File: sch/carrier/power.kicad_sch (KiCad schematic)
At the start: 0 parts

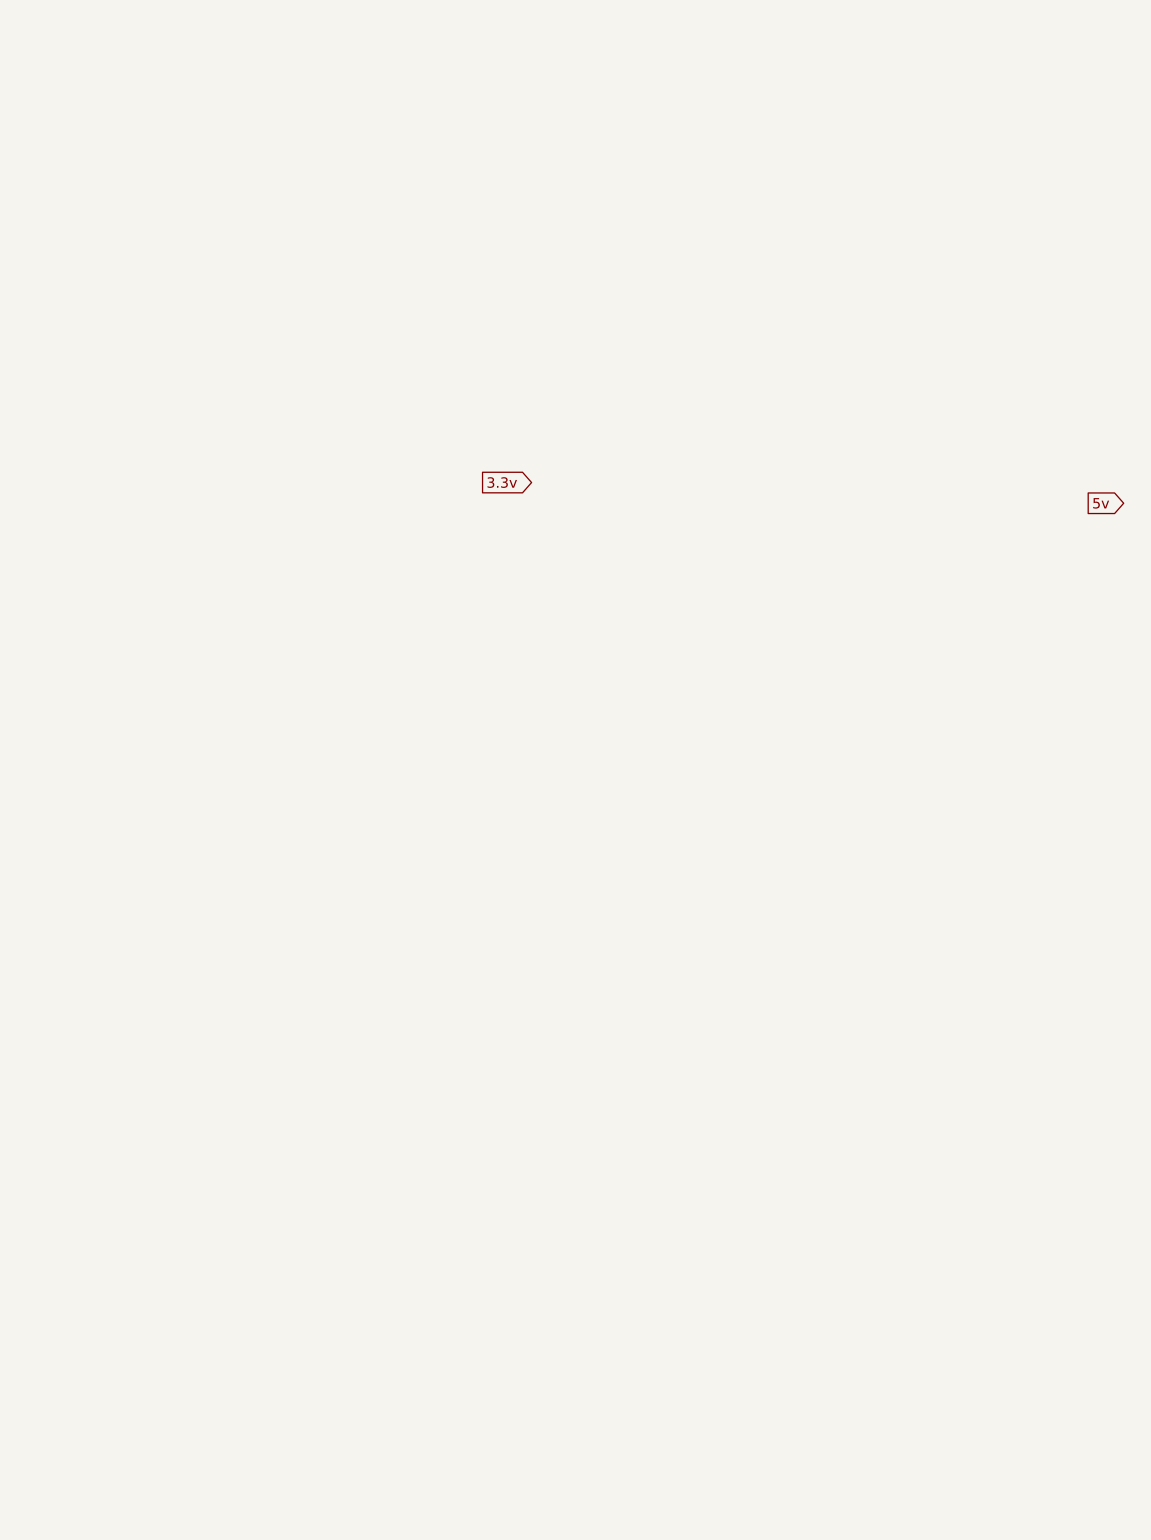
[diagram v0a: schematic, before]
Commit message: noice.
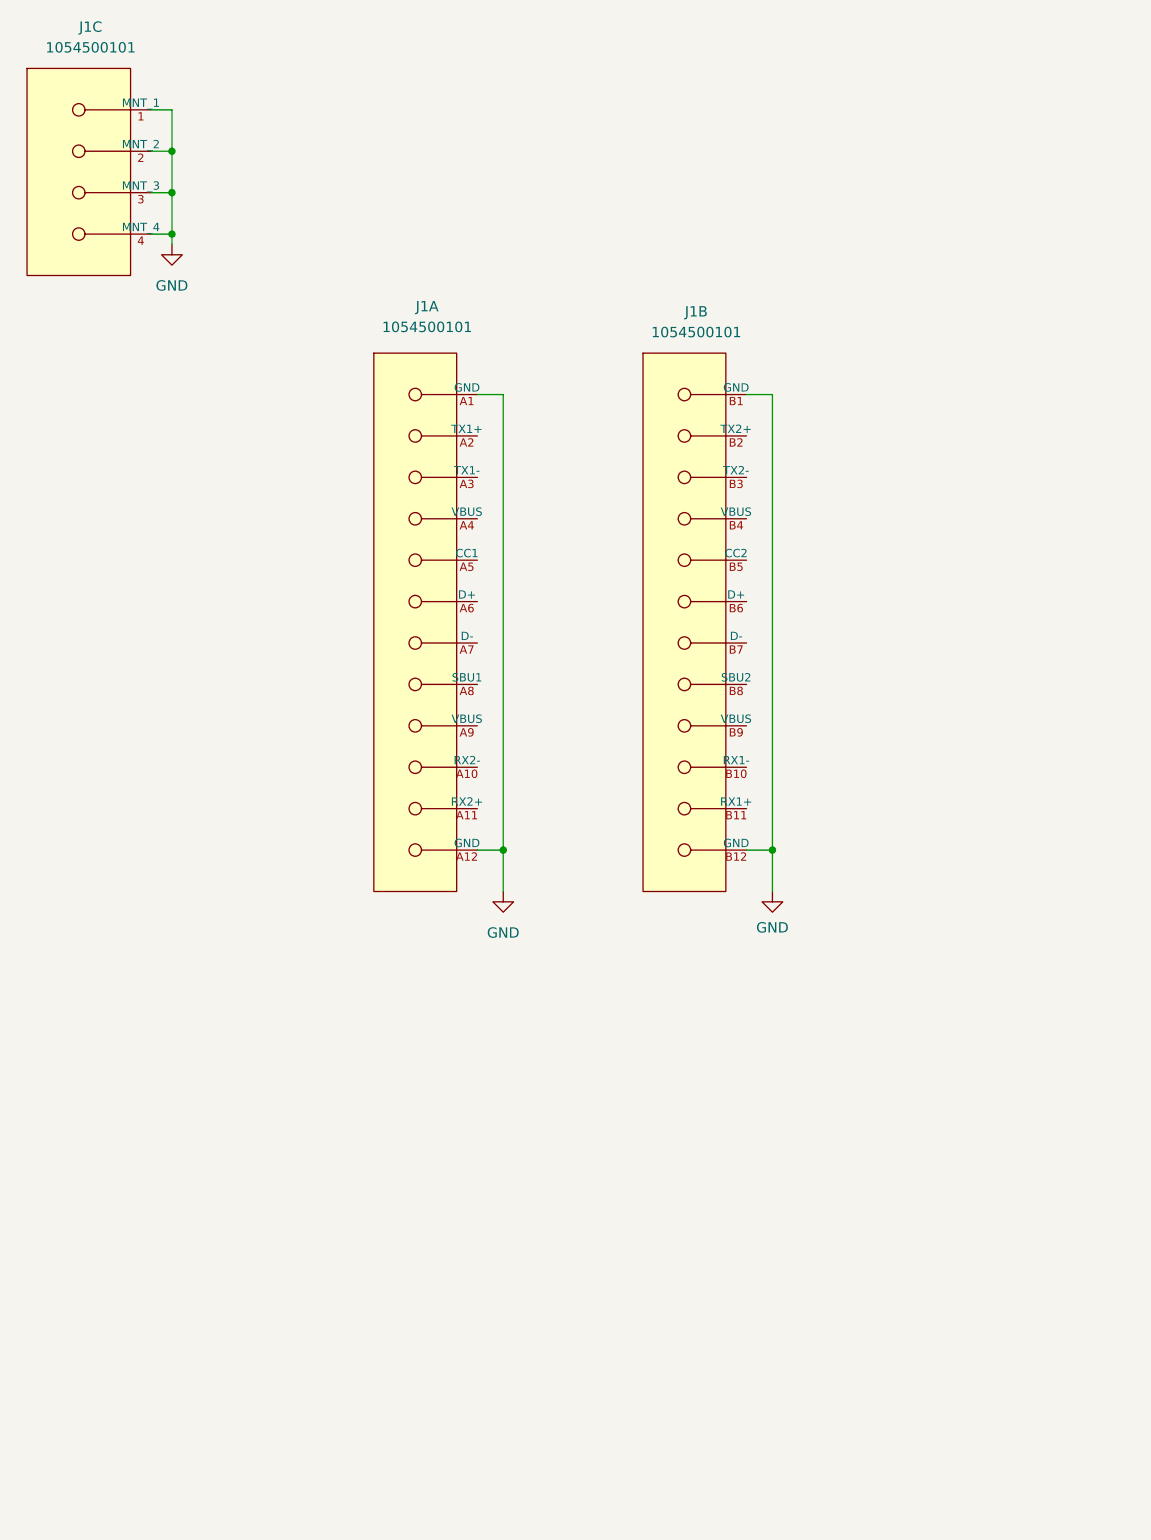
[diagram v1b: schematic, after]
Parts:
- added J1: 1054500101, MOLEXC:Molex-1054500101-MFG, symbol MOLEXC:1054500101
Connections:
- new net GND: J1.1 (MNT_1), J1.2 (MNT_2), J1.3 (MNT_3), J1.4 (MNT_4), J1.A1 (GND), J1.A12 (GND), J1.B1 (GND), J1.B12 (GND)

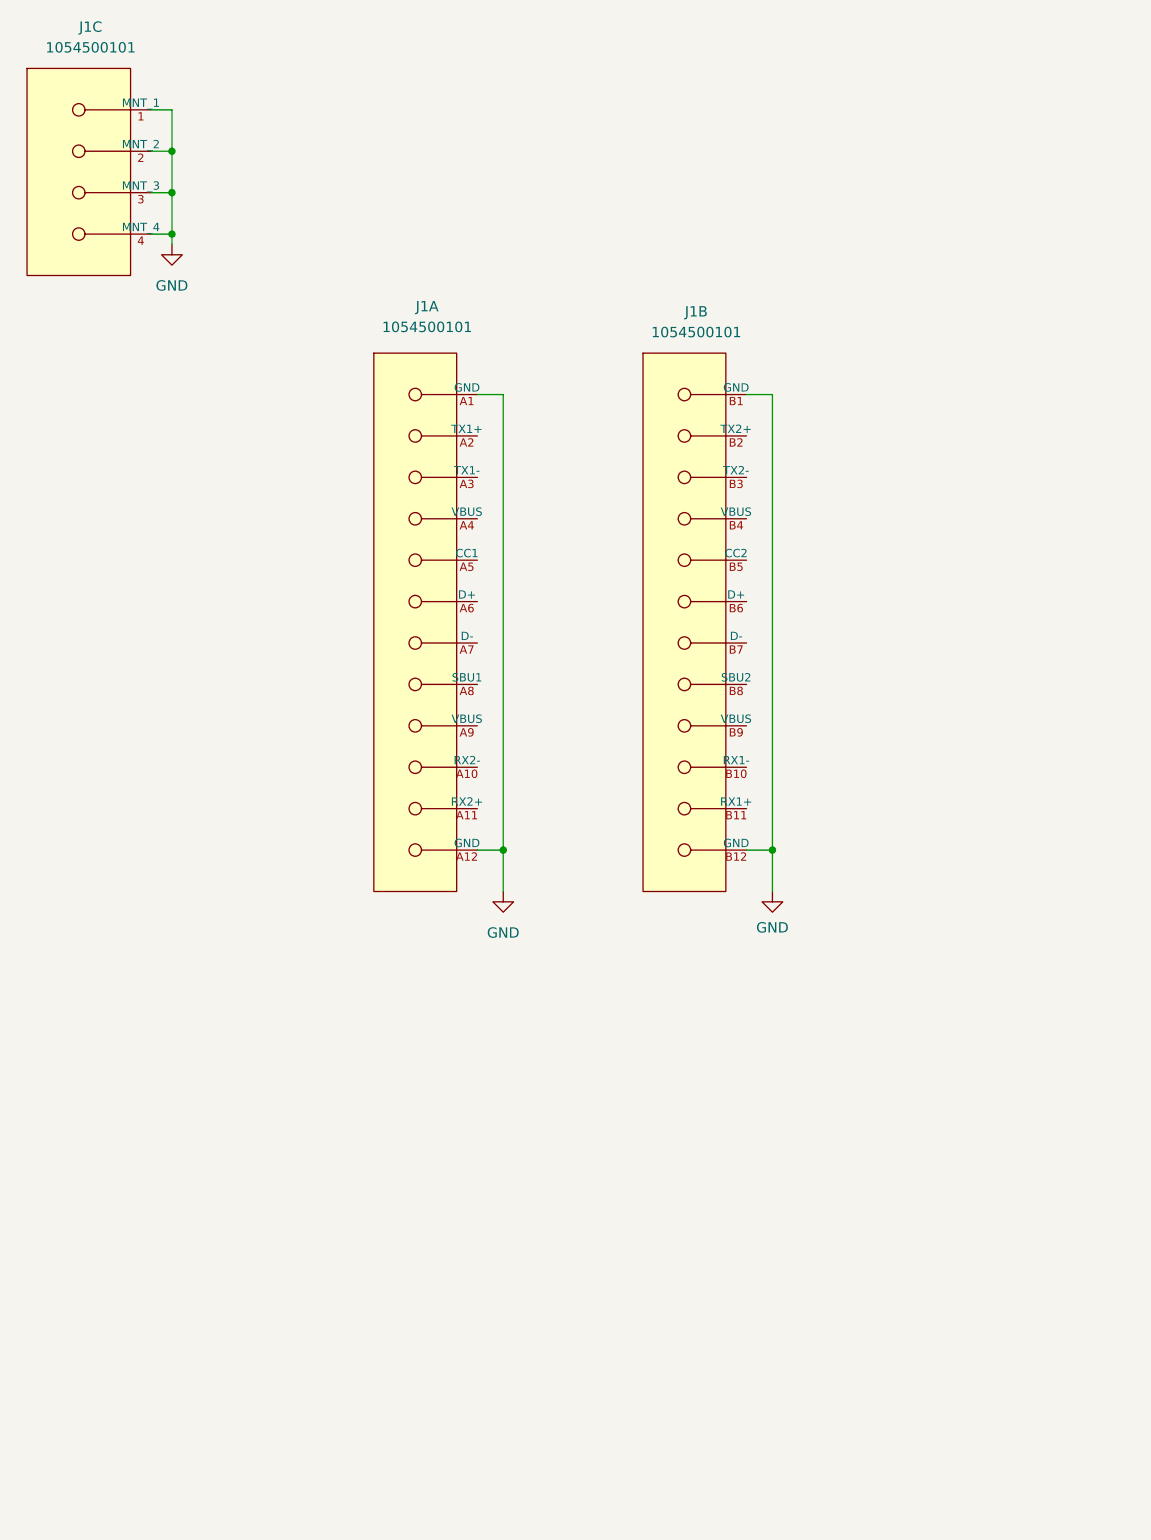
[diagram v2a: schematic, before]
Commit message: goodnight
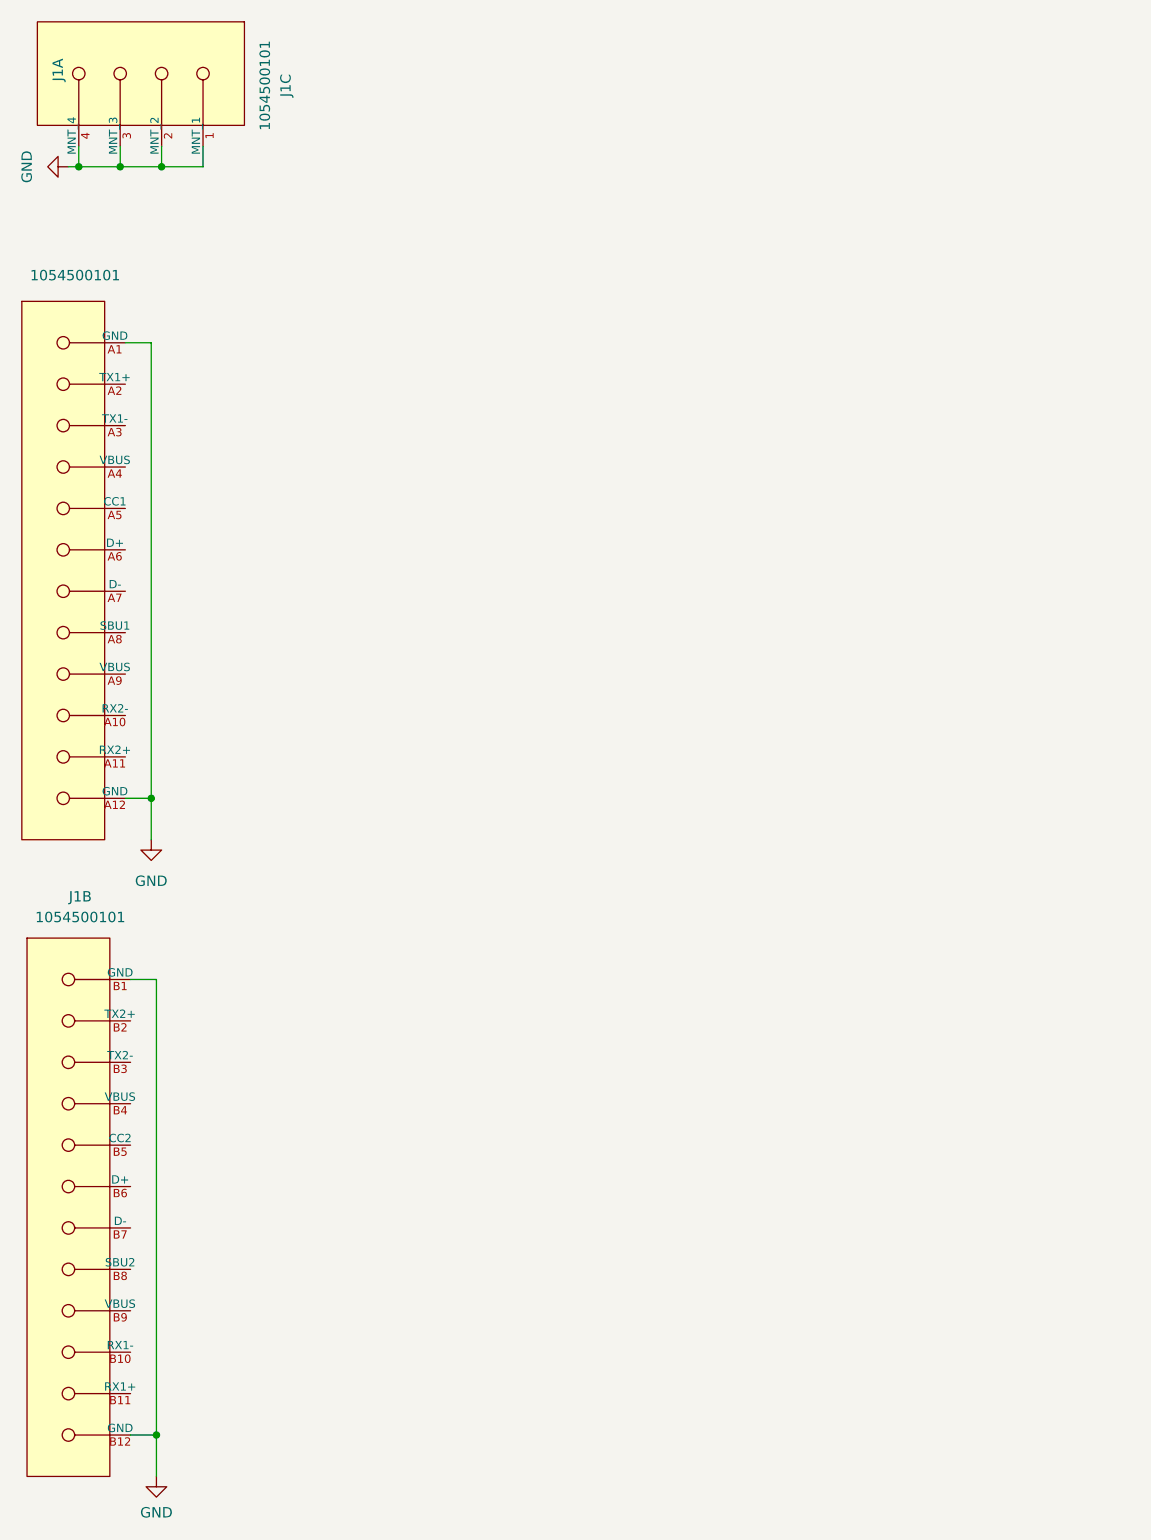
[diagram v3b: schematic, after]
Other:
- title: (none) -> Power and battery
- moved on the sheet: J1A, J1B, J1C

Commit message: hhhhhhhhhhhhhhhhh
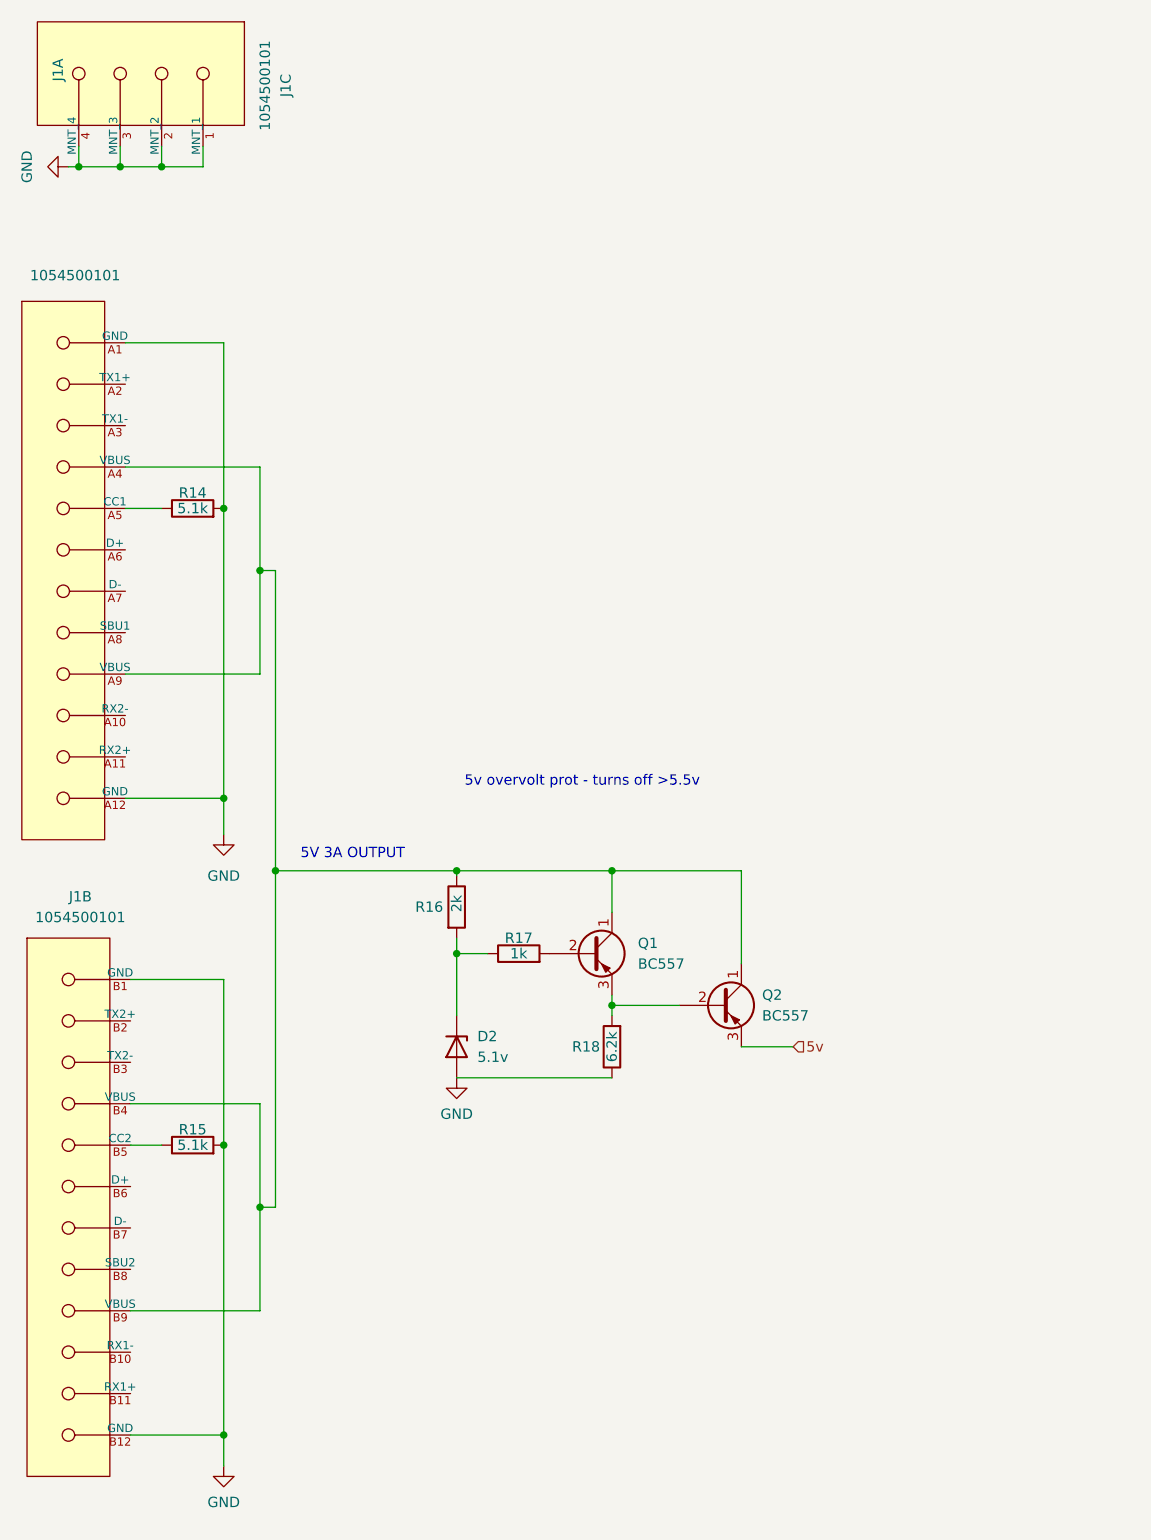
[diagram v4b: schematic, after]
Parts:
- added D2: 5.1v, Diode_THT:D_DO-41_SOD81_P7.62mm_Horizontal, symbol Device:D_Zener
- added Q1, Q2: BC557, Package_TO_SOT_THT:TO-92_Inline, symbol Transistor_BJT:BC557
- added R14, R15: 5.1k, Resistor_SMD:R_0805_2012Metric_Pad1.20x1.40mm_HandSolder, symbol Device:R
- added R16: 2k, Resistor_SMD:R_0805_2012Metric_Pad1.20x1.40mm_HandSolder, symbol Device:R
- added R17: 1k, Resistor_SMD:R_0805_2012Metric_Pad1.20x1.40mm_HandSolder, symbol Device:R
- added R18: 6.2k, Resistor_SMD:R_0805_2012Metric_Pad1.20x1.40mm_HandSolder, symbol Device:R
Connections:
- net GND: now also D2.2 (A), R14.2, R15.2, R18.1
- net at J1.B4 (VBUS): now also J1.A4 (VBUS), J1.A9 (VBUS), J1.B9 (VBUS), Q1.1 (C), Q2.1 (C), R16.1
- net at J1.B5 (CC2): now also R15.1
- net at J1.A5 (CC1): now also R14.1
- new net: D2.1 (K), R16.2, R17.1
- new net: Q1.2 (B), R17.2
- new net: Q1.3 (E), Q2.2 (B), R18.2
- new net 5v: Q2.3 (E)
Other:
- note added: "5V 3A OUTPUT"
- note added: "5v overvolt prot - turns off >5.5v"
